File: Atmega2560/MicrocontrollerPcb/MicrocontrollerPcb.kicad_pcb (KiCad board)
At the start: 2 copper layers, 68.6 x 48.3 mm, 27 parts, among them J1 Conn_02x12_Odd_Even, U1 ATmega2560-16AU

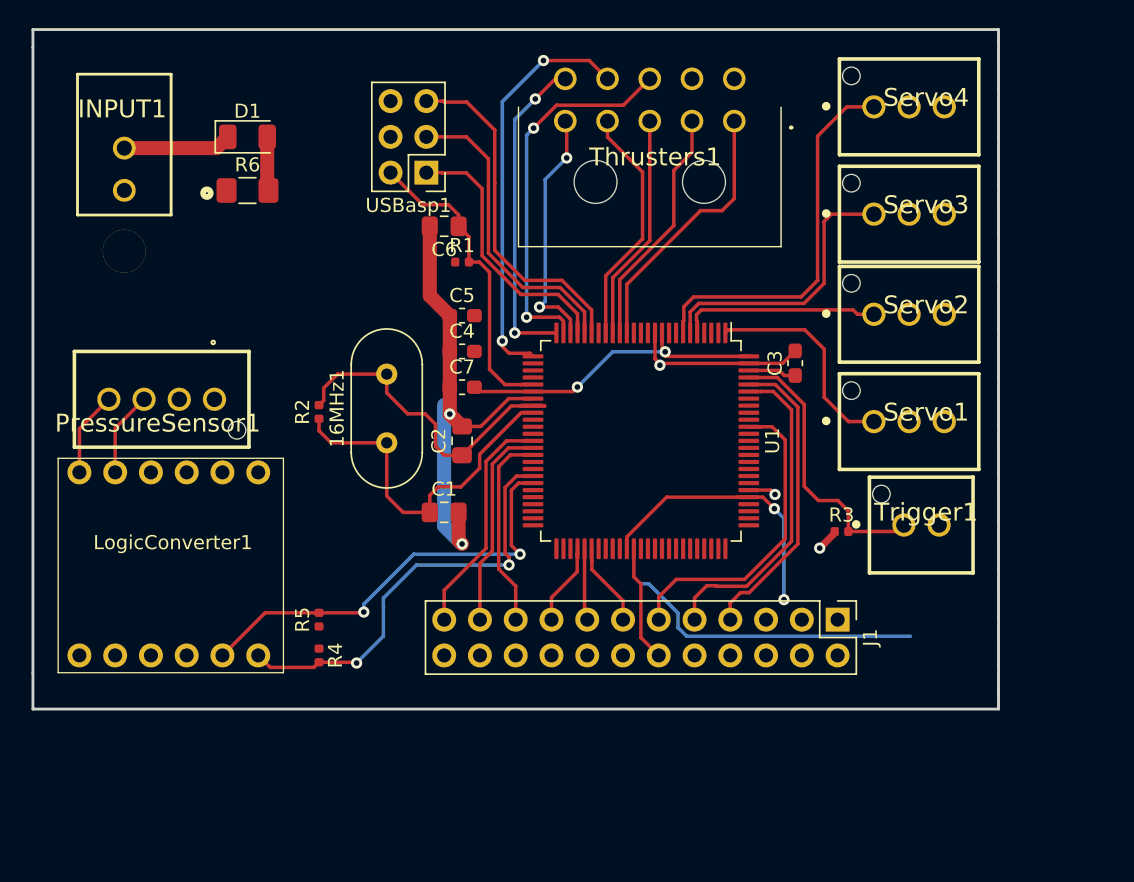
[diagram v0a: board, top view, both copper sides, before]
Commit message: self
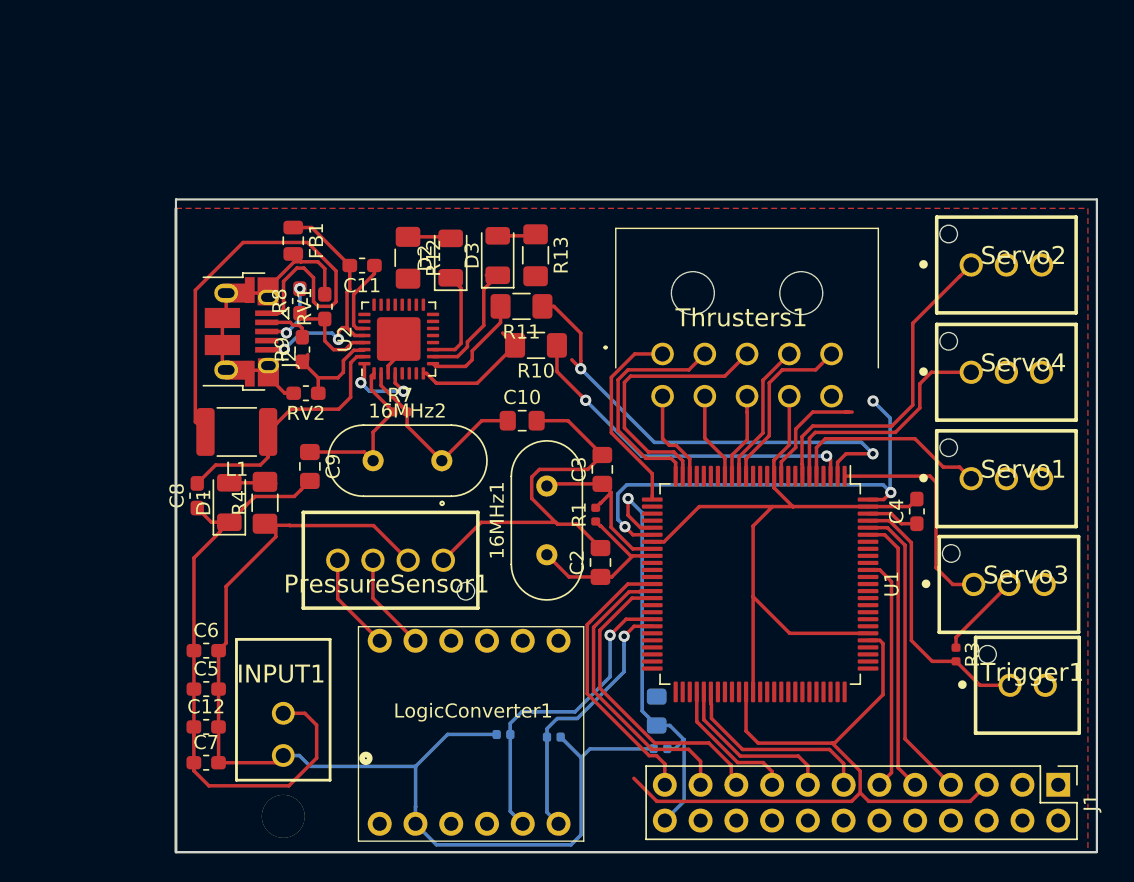
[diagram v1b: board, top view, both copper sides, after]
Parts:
- removed USBasp1: Conn_02x03_Odd_Even, Connector_PinHeader_2.54mm:PinHeader_2x03_P2.54mm_Vertical
- added 16MHz2: Crystal, Crystal:Crystal_HC49-U_Vertical, F.Cu at (157.5, 84.0)
- added C10: 22pF, Capacitor_SMD:C_0805_2012Metric_Pad1.15x1.40mm_HandSolder, F.Cu at (168.1, 81.1)
- added C11: 100n, Capacitor_SMD:C_0603_1608Metric_Pad1.05x0.95mm_HandSolder, F.Cu at (156.7, 70.1)
- added C12: 100n, Capacitor_SMD:C_0603_1608Metric_Pad1.05x0.95mm_HandSolder, F.Cu at (145.7, 102.9)
- added C8: 100n, Capacitor_SMD:C_0603_1608Metric_Pad1.05x0.95mm_HandSolder, F.Cu at (145.0, 86.5)
- added C9: 22pF, Capacitor_SMD:C_0805_2012Metric_Pad1.15x1.40mm_HandSolder, F.Cu at (153.0, 84.4)
- added D2: LED, LED_SMD:LED_1206_3216Metric, F.Cu at (163.0, 69.6)
- added D3: LED, LED_SMD:LED_1206_3216Metric, F.Cu at (166.4, 69.4)
- added FB1: Ferrite_Bead, Resistor_SMD:R_0805_2012Metric, F.Cu at (151.8, 68.3)
- added J2: USB_B_Micro, Connector_USB:USB_Micro-B_Amphenol_10103594-0001LF_Horizontal, F.Cu at (148.2, 74.8)
- added L1: L, Inductor_SMD:L_1812_4532Metric_Pad1.30x3.40mm_HandSolder, F.Cu at (147.8, 81.9)
- added R10: 1K, Resistor_SMD:R_1206_3216Metric_Pad1.42x1.75mm_HandSolder, F.Cu at (169.1, 75.8)
- added R11: 1K, Resistor_SMD:R_1206_3216Metric_Pad1.42x1.75mm_HandSolder, F.Cu at (168.1, 73.0)
- added R12: 1K, Resistor_SMD:R_1206_3216Metric_Pad1.42x1.75mm_HandSolder, F.Cu at (160.0, 69.5)
- added R13: 1K, Resistor_SMD:R_1206_3216Metric_Pad1.42x1.75mm_HandSolder, F.Cu at (169.1, 69.4)
- added R7: 1M, Resistor_SMD:R_0402_1005Metric, F.Cu at (159.4, 80.5)
- added R8: 22R, Resistor_SMD:R_0603_1608Metric_Pad1.05x0.95mm_HandSolder, F.Cu at (152.3, 72.6)
- added R9: 22R, Resistor_SMD:R_0603_1608Metric_Pad1.05x0.95mm_HandSolder, F.Cu at (152.5, 76.1)
- added RV1: Varistor, Resistor_SMD:R_0603_1608Metric_Pad1.05x0.95mm_HandSolder, F.Cu at (154.1, 73.0)
- added RV2: Varistor, Resistor_SMD:R_0603_1608Metric_Pad1.05x0.95mm_HandSolder, F.Cu at (152.7, 79.2)
- added U2: ATmega8U2-MU, Package_DFN_QFN:QFN-32-1EP_5x5mm_P0.5mm_EP3.1x3.1mm, F.Cu at (159.3, 75.3)
- C1, R5: moved to B.Cu
- C3: value 100n -> 22pF; footprint Capacitor_SMD:C_0603_1608Metric_Pad1.05x0.95mm_HandSolder -> Capacitor_SMD:C_0805_2012Metric_Pad1.15x1.40mm_HandSolder
- C6: value 22pF -> 100n; footprint Capacitor_SMD:C_0805_2012Metric_Pad1.15x1.40mm_HandSolder -> Capacitor_SMD:C_0603_1608Metric_Pad1.05x0.95mm_HandSolder
- R1: value 10k -> 1M
- R2: value 1M -> 10k; moved to B.Cu
- R4: value 10K -> 1K; footprint Resistor_SMD:R_0402_1005Metric -> Resistor_SMD:R_1206_3216Metric_Pad1.42x1.75mm_HandSolder
- R6: value 1K -> 10K; footprint Resistor_SMD:R_1206_3216Metric_Pad1.42x1.75mm_HandSolder -> Resistor_SMD:R_0402_1005Metric; moved to B.Cu
- moved R6 44.5 mm to (170.3, 103.6), turned to 180 degrees
- moved INPUT1 41.7 mm to (151.1, 109.2)
- moved C6 34.6 mm to (145.7, 97.5), turned to 0 degrees
- moved C4 34.2 mm to (196.1, 87.6), turned to 90 degrees
- moved R2 34.1 mm to (177.9, 104.4), turned to 0 degrees
- moved C7 32.3 mm to (145.7, 105.4)
- moved C5 32.1 mm to (145.7, 100.2)
- moved Servo3 27.2 mm to (202.7, 96.2)
- moved D1 26.0 mm to (147.3, 86.9), turned to 90 degrees
- moved LogicConverter1 24.5 mm to (170.7, 109.8)
- moved C1 20.7 mm to (177.7, 101.7), turned to 90 degrees
- moved R1 20.3 mm to (173.3, 87.8), turned to 90 degrees
- moved Servo4 20.1 mm to (202.5, 81.1)
- moved PressureSensor1 19.9 mm to (158.8, 87.6)
- moved J1 19.6 mm to (206.2, 107.0)
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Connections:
- C1 pad 1: Net-(16MHz1-Pad1) -> /Reset
- C2 pad 1: Net-(16MHz1-Pad2) -> Net-(16MHz1-Pad1)
- C3 pad 1: Net-(C3-Pad1) -> Net-(16MHz1-Pad2)
- C4 pad 1: Earth -> Net-(C4-Pad1)
- C4 pad 2: +5V -> Earth
- C6 pad 1: /Reset -> Earth
- C6 pad 2: Earth -> +5V
- J1 pad 24: Earth -> /Reset
- LogicConverter1 pad 1: /SCL -> /SDA
- LogicConverter1 pad 2: /SDA -> /SCL
- R1 pad 1: +5V -> Net-(16MHz1-Pad1)
- R1 pad 2: /Reset -> Net-(16MHz1-Pad2)
- R2 pad 1: Net-(16MHz1-Pad1) -> +5V
- R2 pad 2: Net-(16MHz1-Pad2) -> /Reset
- R4 pad 2: /SCL -> Net-(D1-Pad2)
- R5 pad 2: /SDA -> /SCL
- R6 pad 2: Net-(D1-Pad2) -> /SDA
- Servo1 pad 1: Net-(Servo1-Pad1) -> /S2
- Servo2 pad 1: /S2 -> /S4
- Servo3 pad 1: /S3 -> Net-(Servo3-Pad1)
- Servo4 pad 1: /S4 -> /S3
- Thrusters1 pad 10: /T7 -> Earth
- Thrusters1 pad 6: Earth -> /T6
- Thrusters1 pad 7: Earth -> /T7
- Thrusters1 pad 8: /T6 -> /T8
- Thrusters1 pad 9: /T8 -> Earth
- U1 pad 1: Net-(Servo1-Pad1) -> Net-(Servo3-Pad1)
- U1 pad 15: /T1 -> /T5
- U1 pad 16: /T2 -> /T4
- U1 pad 17: /T3 -> /T8
- U1 pad 18: /T4 -> /T7
- U1 pad 2: Net-(U1-Pad2) -> /RX0
- U1 pad 20: /SCK -> Net-(U1-Pad20)
- U1 pad 21: /MOSI -> Net-(U1-Pad21)
- U1 pad 22: /MISO -> Net-(U1-Pad22)
- U1 pad 23: /T5 -> /T6
- U1 pad 24: /T6 -> /T3
- U1 pad 25: /T7 -> /T2
- U1 pad 26: /T8 -> /T1
- U1 pad 3: Net-(U1-Pad3) -> /TX0
- U1 pad 98: Net-(C3-Pad1) -> Net-(C4-Pad1)
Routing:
- net +5V: track 42.1 -> 178.3 mm, vias 4 -> 5
- net Earth: track 86.9 -> 129.6 mm, vias 5 -> 0
- net Net-(J2-Pad1): track 0.00 -> 34.4 mm
- net /RX0: track 0.00 -> 33.9 mm, vias 0 -> 2
- net /TX0: track 0.00 -> 25.5 mm, vias 0 -> 2
- net /SCK: track 24.5 -> 0.00 mm
- net /T8: track 29.1 -> 6.13 mm, vias 2 -> 0
- net Net-(FB1-Pad2): track 0.00 -> 22.7 mm
- net /MOSI: track 21.8 -> 0.00 mm
- net /T6: track 26.9 -> 6.76 mm, vias 2 -> 0
- net /MISO: track 20.1 -> 0.00 mm
- net /USBVCC: track 0.00 -> 19.4 mm
- net Net-(C11-Pad2): track 0.00 -> 18.2 mm, vias 0 -> 2
- net /T7: track 22.9 -> 6.27 mm, vias 2 -> 0
- net Net-(Servo3-Pad1): track 0.00 -> 15.9 mm
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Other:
- board size 68.6 x 48.3 mm -> 65.4 x 46.4 mm
